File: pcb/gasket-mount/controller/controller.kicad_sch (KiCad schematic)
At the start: 36 parts, among them J1 USB_C_Receptacle_USB2.0_16P, U1 USBLC6-2SC6, U4 RP2040, U5 AP2112K-3.3, X1 ABM8-272-T3

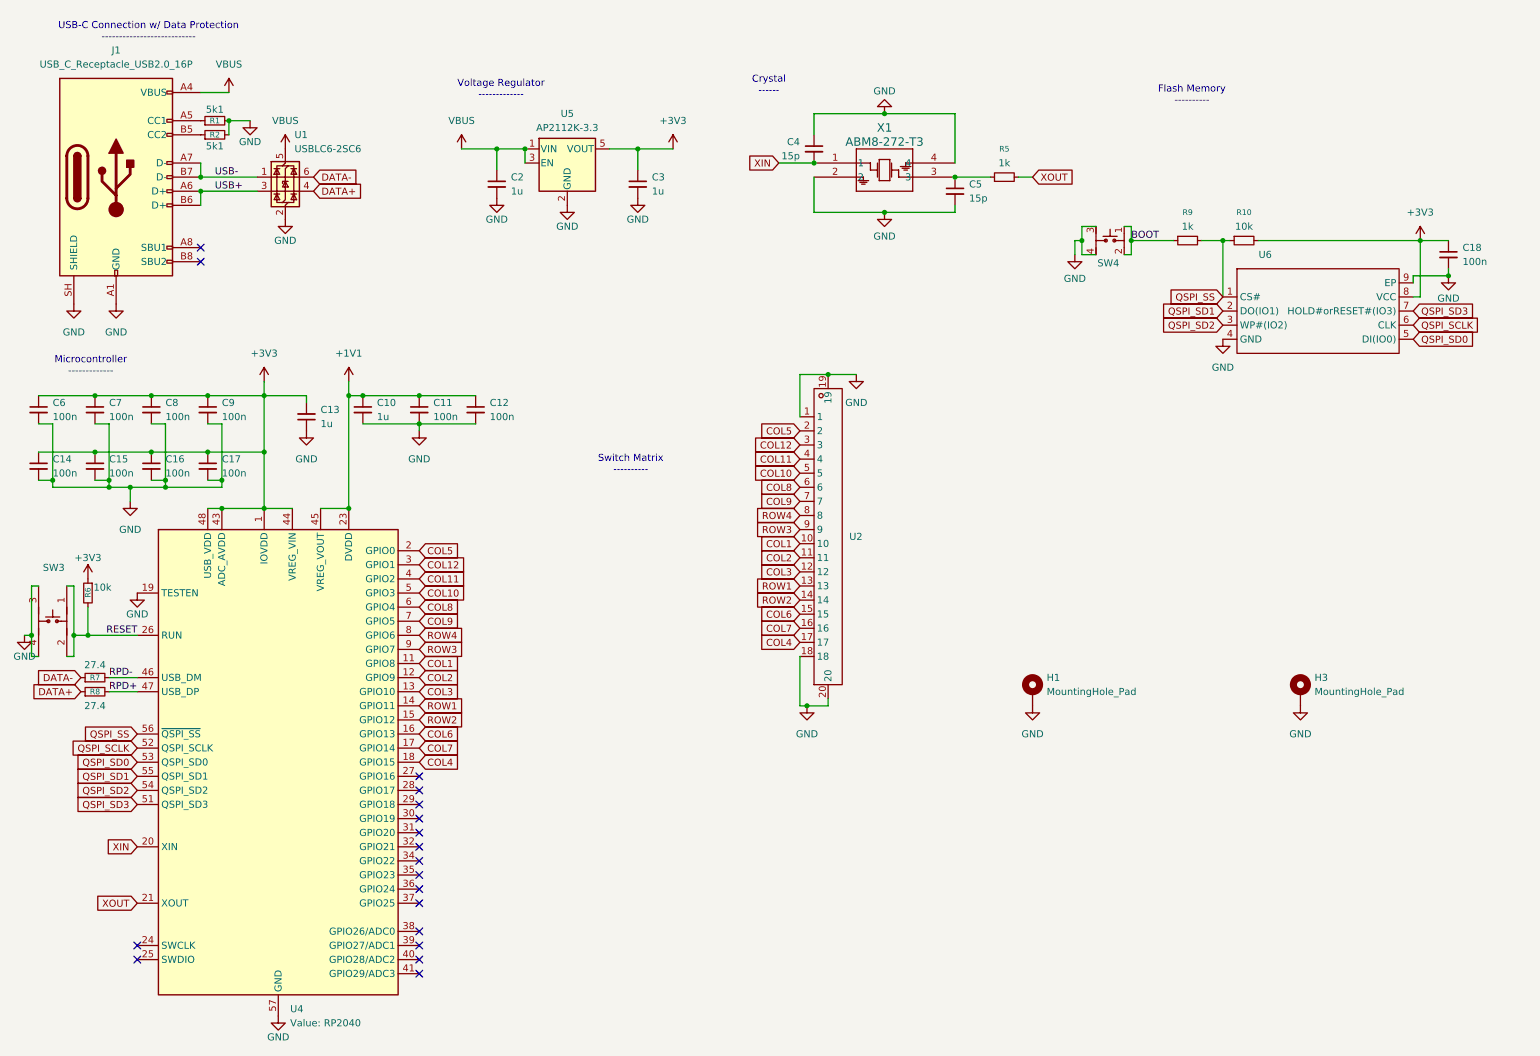
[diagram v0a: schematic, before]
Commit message: PCB finishing touches
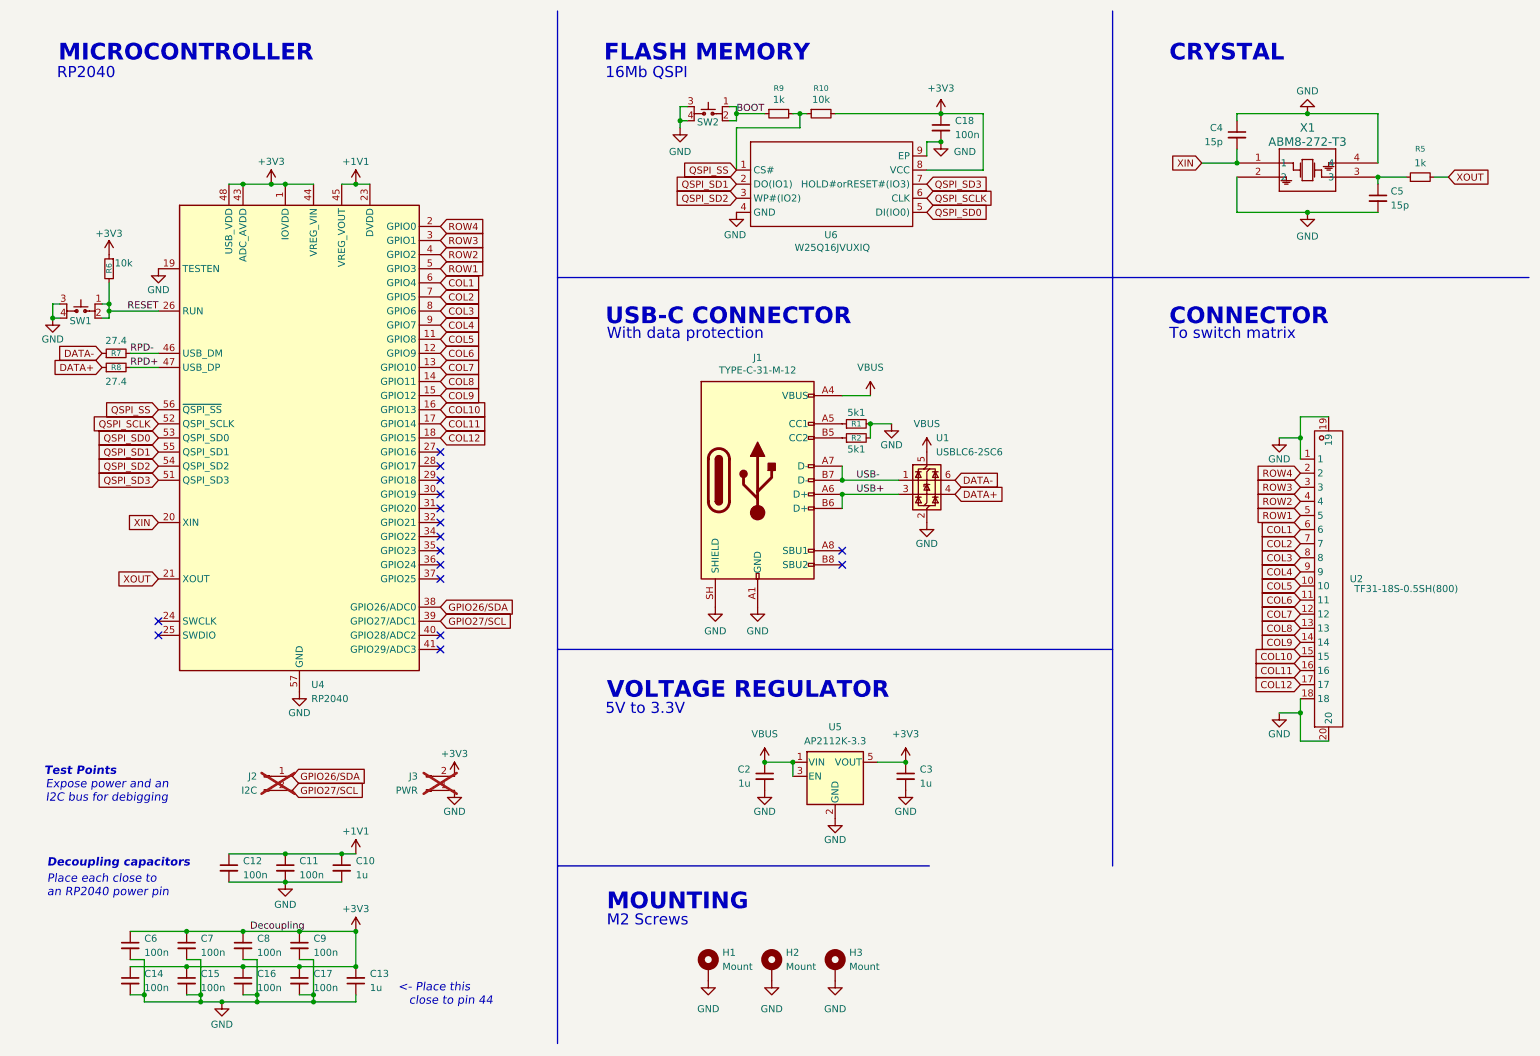
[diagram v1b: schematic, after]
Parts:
- removed SW3: (no value), EasyEDA_Lib:KEY-SMD_4P-L4.2-W3.2-P2.20-LS4.6, symbol EasyEDA_Lib:SKRPAME010
- added H3: Mount, MountingHole:MountingHole_2.2mm_M2_ISO14580_Pad, symbol Mechanical:MountingHole_Pad
- added J2: I2C, Connector_PinHeader_2.54mm:PinHeader_1x02_P2.54mm_Vertical, symbol Connector:Conn_01x02_Pin
- added J3: PWR, Connector_PinHeader_2.54mm:PinHeader_1x02_P2.54mm_Vertical, symbol Connector:Conn_01x02_Pin
- added SW1: (no value), EasyEDA_Lib:KEY-SMD_4P-L4.2-W3.2-P2.20-LS4.6, symbol EasyEDA_Lib:SKRPAME010
- H1: value MountingHole_Pad -> Mount
- H2: renamed from H3; value MountingHole_Pad -> Mount
- J1: value USB_C_Receptacle_USB2.0_16P -> TYPE-C-31-M-12
- U2: value (none) -> TF31-18S-0.5SH(800)
- renumbered SW4 to SW2
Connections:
- net +3V3: now also J3.2 (Pin_2)
- net COL1: now also U2.6, U4.6 (GPIO4); no longer U2.10, U4.11 (GPIO8)
- net COL10: now also U2.15, U4.16 (GPIO13); no longer U2.5, U4.5 (GPIO3)
- net COL11: now also U2.16, U4.17 (GPIO14); no longer U2.4, U4.4 (GPIO2)
- net COL12: now also U2.17, U4.18 (GPIO15); no longer U2.3, U4.3 (GPIO1)
- net COL2: now also U2.7, U4.7 (GPIO5); no longer U2.11, U4.12 (GPIO9)
- net COL3: now also U2.8, U4.8 (GPIO6); no longer U2.12, U4.13 (GPIO10)
- net COL4: now also U2.9, U4.9 (GPIO7); no longer U2.17, U4.18 (GPIO15)
- net COL5: now also U2.10, U4.11 (GPIO8); no longer U2.2, U4.2 (GPIO0)
- net COL6: now also U2.11, U4.12 (GPIO9); no longer U2.15, U4.16 (GPIO13)
- net COL7: now also U2.12, U4.13 (GPIO10); no longer U2.16, U4.17 (GPIO14)
- net COL8: now also U2.13, U4.14 (GPIO11); no longer U2.6, U4.6 (GPIO4)
- net COL9: now also U2.14, U4.15 (GPIO12); no longer U2.7, U4.7 (GPIO5)
- net GND: now also H3.1, J3.1 (Pin_1), SW1.3, SW1.4
- net RESET: now also SW1.1, SW1.2
- net ROW1: now also U2.5, U4.5 (GPIO3); no longer U2.13, U4.14 (GPIO11)
- net ROW2: now also U2.4, U4.4 (GPIO2); no longer U2.14, U4.15 (GPIO12)
- net ROW3: now also U2.3, U4.3 (GPIO1); no longer U2.9, U4.9 (GPIO7)
- net ROW4: now also U2.2, U4.2 (GPIO0); no longer U2.8, U4.8 (GPIO6)
- net GPIO26/SDA: now reaches U4.38 (GPIO26/ADC0)
- net GPIO26/SDA: now also J2.1 (Pin_1)
- net GPIO27/SCL: now reaches U4.39 (GPIO27/ADC1)
- net GPIO27/SCL: now also J2.2 (Pin_2)
- no-connect marks 18 -> 16
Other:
- note added: "16Mb QSPI"
- note added: "5V to 3.3V"
- note added: "<- Place this close to pin 44"
- note added: "CONNECTOR"
- note added: "CRYSTAL"
- note added: "Decoupling capacitors"
- note added: "Expose power and an I2C bus for debigging"
- note added: "FLASH MEMORY"
- note added: "M2 Screws"
- note added: "MICROCONTROLLER"
- note added: "MOUNTING"
- note added: "Place each close to an RP2040 power pin"
- note added: "RP2040"
- note added: "Test Points"
- note added: "To switch matrix"
- note added: "USB-C CONNECTOR"
- note added: "VOLTAGE REGULATOR"
- note added: "With data protection"
- note removed: "Crystal ------"
- note removed: "Flash Memory ----------"
- note removed: "Microcontroller -------------"
- note removed: "Switch Matrix ----------"
- note removed: "USB-C Connection w/ Data Protection ---------------------------"
- note removed: "Voltage Regulator -------------"
- moved on the sheet: C10, C11, C12, C13, C14, C15, C16, C17, C18, C2, C3, C4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
